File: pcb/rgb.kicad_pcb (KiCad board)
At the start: 2 copper layers, 128 x 30 mm, 22 parts, among them J1 Conn_02x08_Odd_Even, J2 Conn_01x02, J3 Conn_01x02, P1 TTL_232R_3V3, U1 ESP-WROOM-32, U2 REG1117, U3 412D02F, U4 TACTILE, U5 TACTILE, U6 MicroSD_SPI_CD

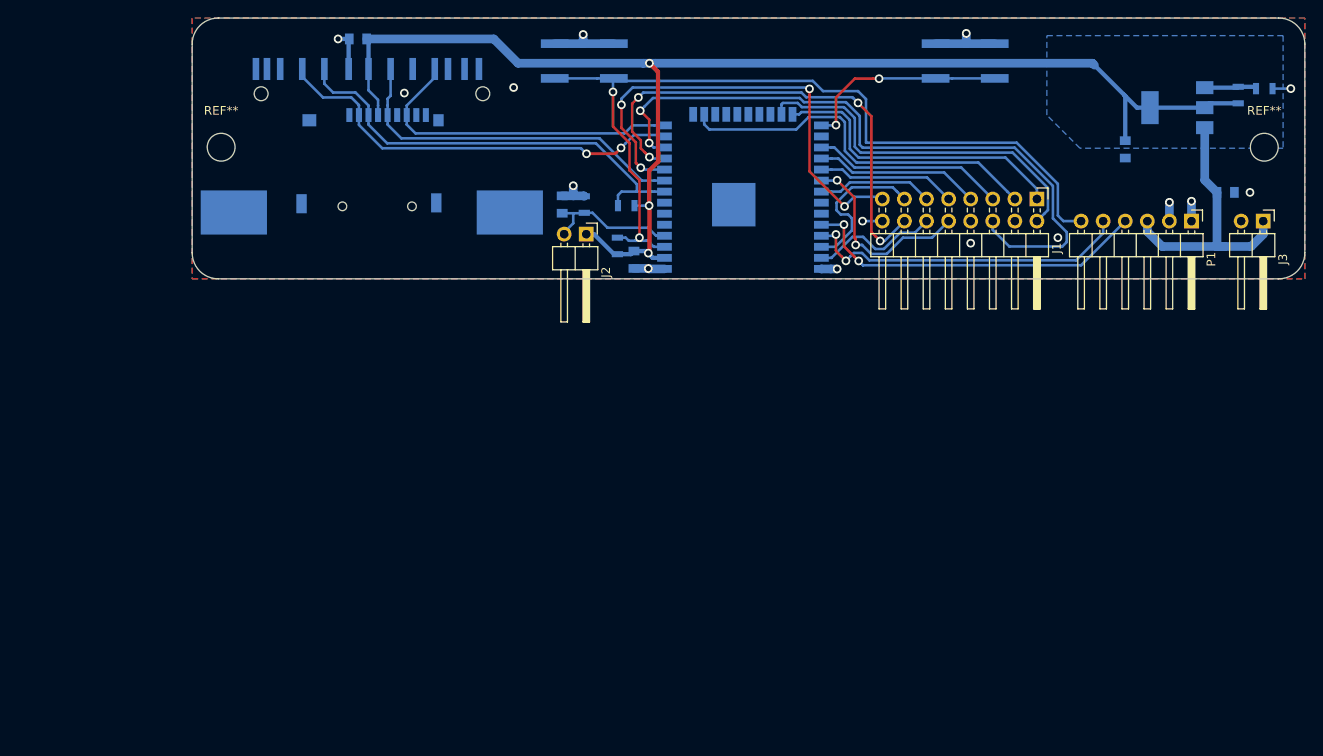
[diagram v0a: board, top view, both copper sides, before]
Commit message: pcb: exploration
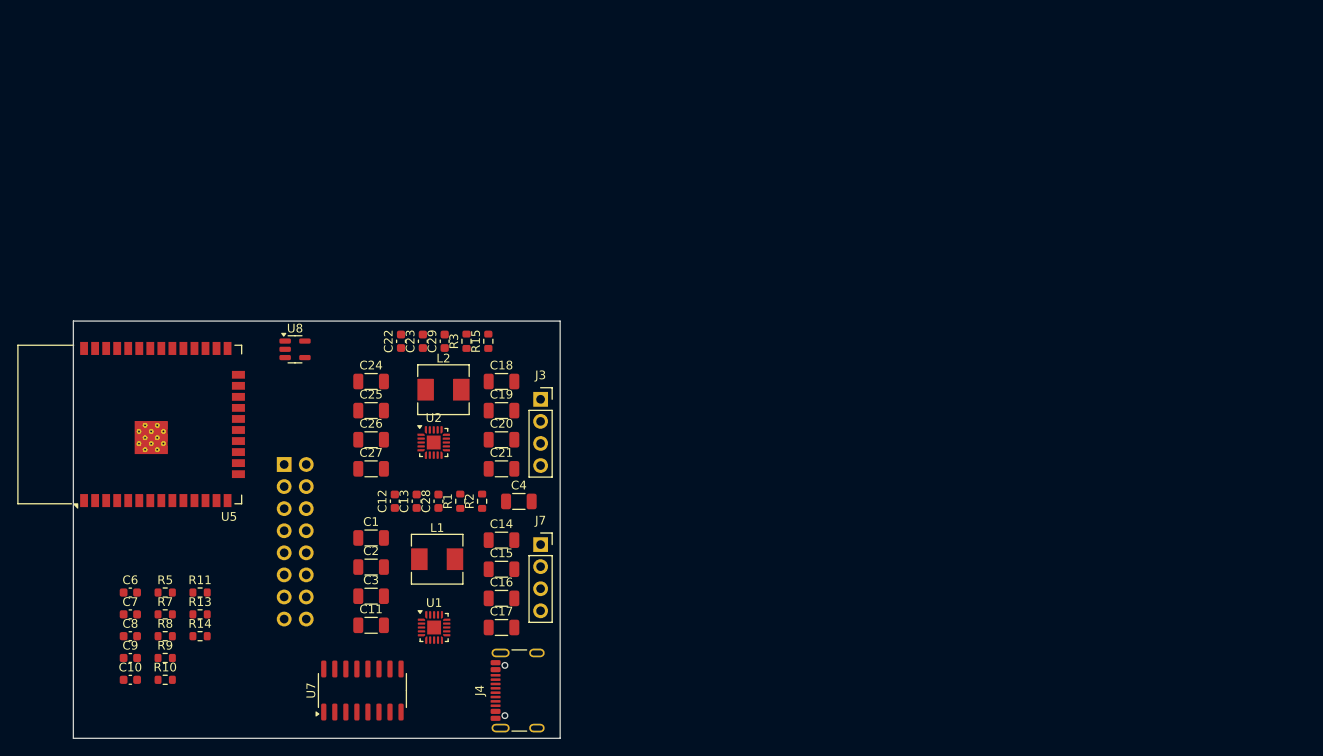
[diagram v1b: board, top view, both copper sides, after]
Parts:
- removed C5: 1u, Capacitors_SMD:C_0805
- removed J2: Conn_01x02, Pin_Headers:Pin_Header_Angled_1x02_Pitch2.54mm
- removed P1: TTL_232R_3V3, Pin_Headers:Pin_Header_Angled_1x06_Pitch2.54mm
- removed R4, R6: 10k, Resistors_SMD:R_0805
- removed REF** (x2): MountingHole_3.2mm_M3, Mounting_Holes:MountingHole_3.2mm_M3
- removed U3: 412D02F, myStuff:RPIA_SD_CARD
- removed U4: TACTILE, myStuff:EVQQ2
- removed U6: MicroSD_SPI_CD, newStuff:GCT-MEM2055-00-190-01-A
- added C10: 2u2, Capacitor_SMD:C_0603_1608Metric, F.Cu at (52.6, 116.3)
- added C11: 10u, Capacitor_SMD:C_1206_3216Metric, F.Cu at (80.2, 110.0)
- added C12: 2u2, Capacitor_SMD:C_0603_1608Metric, F.Cu at (83.0, 95.7)
- added C13: 2u2, Capacitor_SMD:C_0603_1608Metric, F.Cu at (85.5, 95.7)
- added C14: 10u, Capacitor_SMD:C_1206_3216Metric, F.Cu at (95.2, 100.2)
- added C15: 10u, Capacitor_SMD:C_1206_3216Metric, F.Cu at (95.2, 103.5)
- added C16: 10u, Capacitor_SMD:C_1206_3216Metric, F.Cu at (95.2, 106.9)
- added C17: 10u, Capacitor_SMD:C_1206_3216Metric, F.Cu at (95.2, 110.2)
- added C18: 10u, Capacitor_SMD:C_1206_3216Metric, F.Cu at (95.2, 82.0)
- added C19: 10u, Capacitor_SMD:C_1206_3216Metric, F.Cu at (95.2, 85.3)
- added C20: 10u, Capacitor_SMD:C_1206_3216Metric, F.Cu at (95.2, 88.7)
- added C21: 10u, Capacitor_SMD:C_1206_3216Metric, F.Cu at (95.2, 92.0)
- added C22: 2u2, Capacitor_SMD:C_0603_1608Metric, F.Cu at (83.7, 77.3)
- added C23: 2u2, Capacitor_SMD:C_0603_1608Metric, F.Cu at (86.2, 77.3)
- added C24: 10u, Capacitor_SMD:C_1206_3216Metric, F.Cu at (80.2, 82.0)
- added C25: 10u, Capacitor_SMD:C_1206_3216Metric, F.Cu at (80.2, 85.3)
- added C26: 10u, Capacitor_SMD:C_1206_3216Metric, F.Cu at (80.2, 88.7)
- added C27: 10u, Capacitor_SMD:C_1206_3216Metric, F.Cu at (80.2, 92.0)
- added C28: 2u2, Capacitor_SMD:C_0603_1608Metric, F.Cu at (88.0, 95.7)
- added C29: 2u2, Capacitor_SMD:C_0603_1608Metric, F.Cu at (88.7, 77.3)
- added C6: 2u2, Capacitor_SMD:C_0603_1608Metric, F.Cu at (52.6, 106.2)
- added C7: 2u2, Capacitor_SMD:C_0603_1608Metric, F.Cu at (52.6, 108.7)
- added C8: 2u2, Capacitor_SMD:C_0603_1608Metric, F.Cu at (52.6, 111.2)
- added C9: 2u2, Capacitor_SMD:C_0603_1608Metric, F.Cu at (52.6, 113.8)
- added J4: TYPE-C-31-M-12, Connector_USB:USB_C_Receptacle_GCT_USB4105-xx-A_16P_TopMnt_Horizontal, F.Cu at (98.2, 117.5)
- added J7: B4PS-VH, Connector_PinSocket_2.54mm:PinSocket_1x04_P2.54mm_Vertical, F.Cu at (99.8, 100.7)
- added L1: 3u3, Inductor_SMD:L_Sunlord_MWSA0503S, F.Cu at (87.8, 102.4)
- added L2: 3u3, Inductor_SMD:L_Sunlord_MWSA0503S, F.Cu at (88.6, 82.9)
- added R10: 57k, Resistor_SMD:R_0603_1608Metric, F.Cu at (56.6, 116.3)
- added R11: 10k, Resistor_SMD:R_0603_1608Metric, F.Cu at (60.6, 106.2)
- added R13: 22k, Resistor_SMD:R_0603_1608Metric, F.Cu at (60.6, 108.7)
- added R14: 22k, Resistor_SMD:R_0603_1608Metric, F.Cu at (60.6, 111.2)
- added R15: 1k37, Resistor_SMD:R_0603_1608Metric, F.Cu at (93.7, 77.3)
- added R5: 37k4, Resistor_SMD:R_0603_1608Metric, F.Cu at (56.6, 106.2)
- added R7: 22k, Resistor_SMD:R_0603_1608Metric, F.Cu at (56.6, 108.7)
- added R8: 1k, Resistor_SMD:R_0603_1608Metric, F.Cu at (56.6, 111.2)
- added R9: 10k, Resistor_SMD:R_0603_1608Metric, F.Cu at (56.6, 113.8)
- added U7: CH340C, Package_SO:SOIC-16_3.9x9.9mm_P1.27mm, F.Cu at (79.2, 117.5)
- added U8: SPX3819M5-L, Package_TO_SOT_SMD:SOT-23-5, F.Cu at (71.5, 78.2)
- C1: value 470n -> 10u; footprint Capacitors_SMD:C_0805 -> Capacitor_SMD:C_1206_3216Metric; moved to F.Cu
- C2, C3, C4: footprint Capacitors_SMD:C_0805 -> Capacitor_SMD:C_1206_3216Metric; moved to F.Cu
- J1: footprint Pin_Headers:Pin_Header_Angled_2x08_Pitch2.54mm -> Connector_PinSocket_2.54mm:PinSocket_2x08_P2.54mm_Vertical; moved to B.Cu
- J3: value Conn_01x02 -> B4PS-VH; footprint Pin_Headers:Pin_Header_Angled_1x02_Pitch2.54mm -> Connector_PinSocket_2.54mm:PinSocket_1x04_P2.54mm_Vertical
- R1: value 470k -> 10k; footprint Resistors_SMD:R_0805 -> Resistor_SMD:R_0603_1608Metric; moved to F.Cu
- R2: value 590R -> 1k37; footprint Resistors_SMD:R_0805 -> Resistor_SMD:R_0603_1608Metric; moved to F.Cu
- R3: value 1k -> 10k; footprint Resistors_SMD:R_0805 -> Resistor_SMD:R_0603_1608Metric; moved to F.Cu
- U1: value ESP-WROOM-32 -> SY8286ARAC; footprint myStuff:ESP-WROOM-32 -> Package_DFN_QFN:QFN-20-1EP_3x3mm_P0.45mm_EP1.6x1.6mm; moved to F.Cu
- U2: value REG1117 -> SY8286ARAC; footprint SOT-223 -> Package_DFN_QFN:QFN-20-1EP_3x3mm_P0.45mm_EP1.6x1.6mm; moved to F.Cu
- U5: value TACTILE -> ESP32-WROOM-32E; footprint myStuff:EVQQ2 -> RF_Module:ESP32-WROOM-32D; moved to F.Cu
- moved C3 108.7 mm to (80.2, 106.7), turned to 0 degrees
- moved U5 102.1 mm to (55.5, 86.9), turned to 90 degrees
- moved C2 99.2 mm to (80.2, 103.3), turned to 0 degrees
- moved R2 98.7 mm to (93.0, 95.7)
- moved R3 96.3 mm to (91.2, 77.3), turned to 90 degrees
- moved U2 93.8 mm to (87.5, 89.0), turned to 0 degrees
- moved J1 91.8 mm to (70.2, 91.5), turned to 180 degrees
- moved J3 85.6 mm to (99.8, 84.0), turned to 0 degrees
- moved C4 56.3 mm to (97.2, 95.8), turned to 0 degrees
- moved U1 49.0 mm to (87.5, 110.2)
- moved C1 44.0 mm to (80.2, 100.0), turned to 0 degrees
- moved R1 34.5 mm to (90.5, 95.7)
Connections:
- C1 pad 2: +3V3 -> VBUS
- C2 pad 2: +3V3 -> VBUS
- C3 pad 2: +5V -> VBUS
- J3 pad 1: +5V -> /Stepdown_b/v_out
- J3 pad 2: GND -> /Stepdown_b/v_out
- R1 pad 1: +3V3 -> +5V
- R1 pad 2: /rstBtn -> Net-(U1-FB)
- R2 pad 1: +3V3 -> Net-(U1-FB)
- R2 pad 2: Net-(R2-Pad2) -> GND
- R3 pad 1: Net-(R2-Pad2) -> /Stepdown_b/v_out
- R3 pad 2: GND -> Net-(U2-FB)
- U1 pad 1: GND -> Net-(C13-K)
- U1 pad 10: /OE -> unconnected-(U1-NC-Pad10)
- U1 pad 11: /STB -> VBUS
- U1 pad 12: /G1 -> GND
- U1 pad 13: /SD_CS -> unconnected-(U1-ILMT-Pad13)
- U1 pad 14: /SD_MISO -> Net-(U1-FB)
- U1 pad 15: GND -> Net-(C28-A)
- U1 pad 16: /B0 -> unconnected-(U1-NC-Pad16)
- U1 pad 18: Net-(U1-Pad18) -> GND
- U1 pad 19: Net-(U1-Pad19) -> Net-(C13-A)
- U1 pad 2: +3V3 -> VBUS
- U1 pad 20: Net-(U1-Pad20) -> Net-(C13-A)
- U1 pad 21: Net-(U1-Pad21) -> GND
- U1 pad 3: /rstBtn -> VBUS
- U1 pad 4: Net-(C5-Pad1) -> VBUS
- U1 pad 5: Net-(U1-Pad5) -> VBUS
- U1 pad 6: Net-(U1-Pad6) -> Net-(C13-A)
- U1 pad 7: Net-(U1-Pad7) -> GND
- U1 pad 8: /SD_MOSI -> GND
- U1 pad 9: /SD_CLK -> unconnected-(U1-PG-Pad9)
- U2 pad 1: Net-(R2-Pad2) -> Net-(C23-K)
- U2 pad 2: +3V3 -> VBUS
- U2 pad 3: +5V -> VBUS
- U2 pad 4: +3V3 -> VBUS
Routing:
- net +3V3: track 153.5 -> 0.00 mm, vias 3 -> 0
- net /rstBtn: track 98.5 -> 0.00 mm, vias 2 -> 0
- net /G1: track 78.0 -> 0.00 mm, vias 2 -> 0
- net /STB: track 56.5 -> 0.00 mm, vias 4 -> 0
- net /OE: track 54.0 -> 0.00 mm, vias 4 -> 0
- net /SD_MOSI: track 51.3 -> 0.00 mm
- net /SD_CS: track 48.5 -> 0.00 mm, vias 2 -> 0
- net /B0: track 43.6 -> 0.00 mm
- net /G0: track 42.2 -> 0.00 mm
- net /SD_CLK: track 41.1 -> 0.00 mm
- net Net-(P1-Pad4): track 40.5 -> 0.00 mm, vias 2 -> 0
- net GND: track 38.5 -> 0.00 mm, vias 15 -> 0
- net Net-(P1-Pad5): track 38.3 -> 0.00 mm, vias 2 -> 0
- net /SD_MISO: track 38.2 -> 0.00 mm
- net /R0: track 35.0 -> 0.00 mm
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- removed copper zone on B.Cu, net +3V3
- removed copper zone on B.Cu, net GND
- removed copper zone on F.Cu, net GND
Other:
- board size 128 x 30 mm -> 56 x 48 mm
- net class Default removed
- board text removed: "5V"
- board text removed: "Espirgbani"
- board text removed: "FLASH"
- board text removed: "LED panel"
- board text removed: "RESET"
- board text removed: "Rev 1, 02/2018"
- board text removed: "Sens"
- board text removed: "UART"
